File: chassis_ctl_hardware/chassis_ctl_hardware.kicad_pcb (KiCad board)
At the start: 2 copper layers, 75 x 75 mm, 53 parts, among them IC1 TJA1441AT, J1 USB_C, J2 Conn_01x05_Socket, J3 encoder1, J4 encoder2, J5 Conn_01x04_Socket, J6 RJ45, J7 STLink-v3mini, SW1 SW_Push, U1 BU33SD5WG-TR, U2 ICM-40609-D, U3 STM32U545CET6, Y1 16M

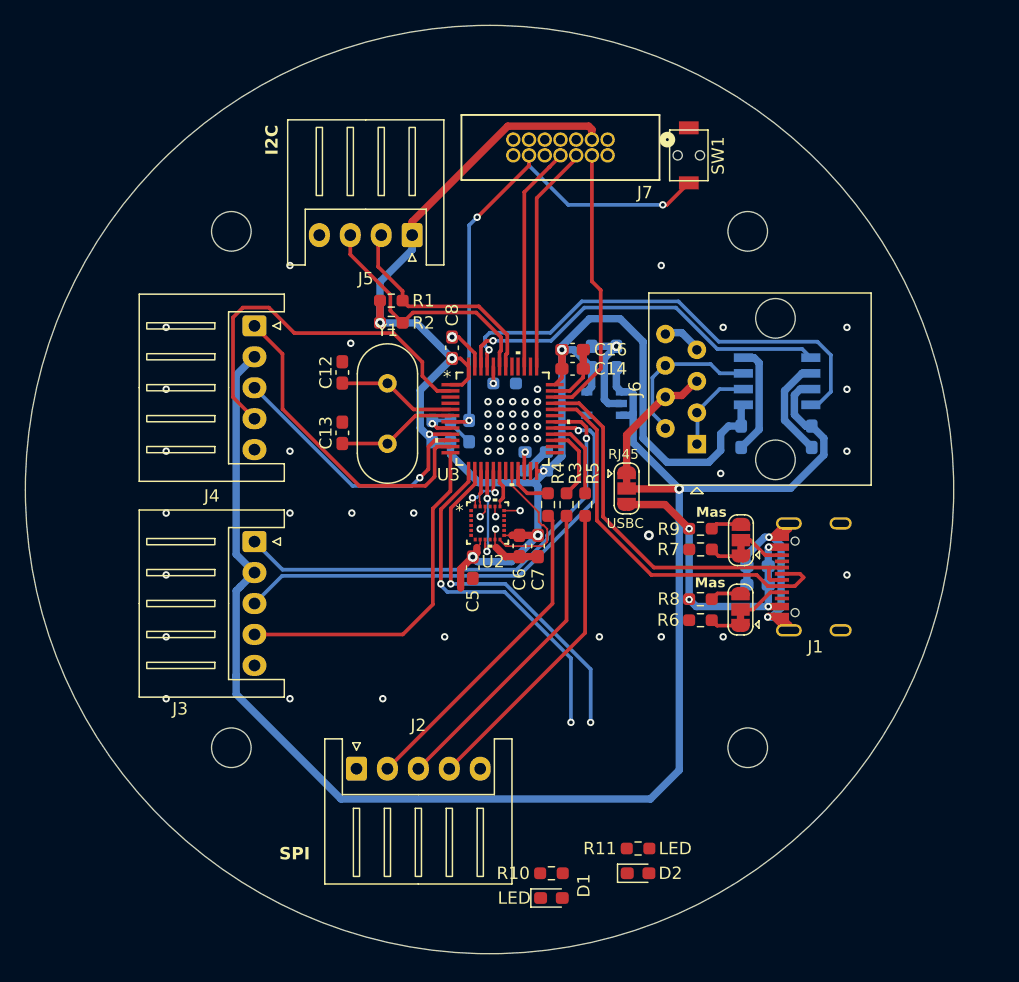
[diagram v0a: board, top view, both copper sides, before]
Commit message: Second_Commit
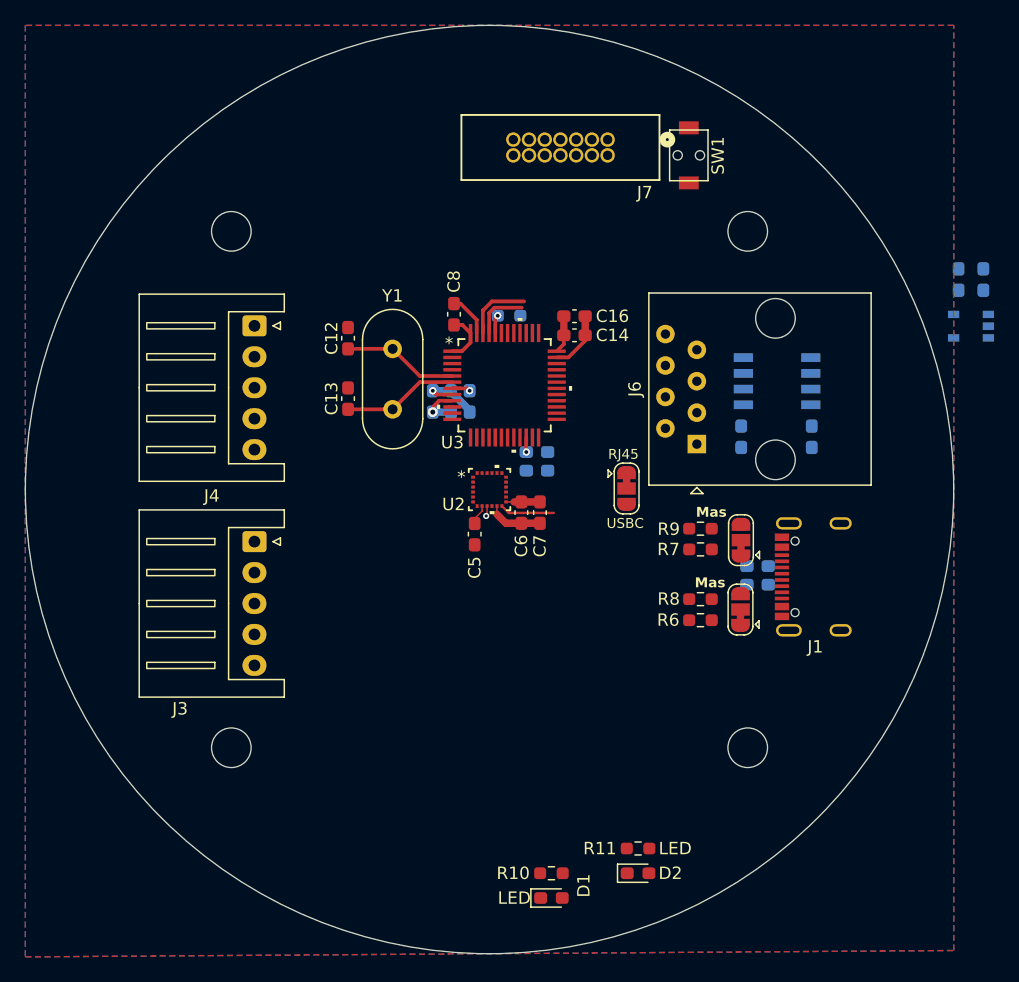
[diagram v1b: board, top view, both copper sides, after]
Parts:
- removed J2: Conn_01x05_Socket, Connector_JST:JST_XH_S5B-XH-A_1x05_P2.50mm_Horizontal
- removed J5: Conn_01x04_Socket, Connector_JST:JST_XH_S4B-XH-A_1x04_P2.50mm_Horizontal
- removed R1, R2: 4.7k, Resistor_SMD:R_0603_1608Metric_Pad0.98x0.95mm_HandSolder
- removed R3, R4, R5: 0, Resistor_SMD:R_0603_1608Metric_Pad0.98x0.95mm_HandSolder
- moved U1 30.3 mm to (199.4, 57.3)
- moved C3 30.3 mm to (198.4, 53.5)
- moved C4 30.3 mm to (200.4, 53.5)
- moved R12 5.48 mm to (162.1, 56.4)
- moved Y1 2.81 mm to (152.7, 64.0)
- moved C13 2.80 mm to (149.1, 63.1)
- moved C12 2.80 mm to (149.1, 58.3)
- moved C14 2.71 mm to (167.4, 58.0)
- moved C5 2.71 mm to (159.3, 74.1)
- moved U2 2.71 mm to (160.5, 70.5)
- moved C16 2.71 mm to (167.4, 56.5)
- moved C8 2.71 mm to (157.6, 56.3)
- moved U3 2.71 mm to (161.7, 62.1)
- moved C6 2.70 mm to (163.1, 72.3)
- moved C7 2.70 mm to (164.6, 72.3)
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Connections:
- net /TIM1_ETR renamed /TIM2_CH3
- J3 pad 1: /TIM1_CH2 -> /TIM2_CH2
- J3 pad 3: /TIM1_CH1 -> /TIM2_CH1
- J4 pad 1: /TIM2_CH2 -> /TIM3_CH2
- J4 pad 3: /TIM2_CH1 -> /TIM3_CH1
- J4 pad 4: /TIM2_ETR -> /TIM3_CH3
- U3 pad 13: /MCU/MCU_State_LED -> unconnected-(U3-PA3-Pad13)
- U3 pad 14: /MCU/FDCAN_State -> unconnected-(U3-PA4-Pad14)
- U3 pad 15: /IMU/SPI_CLK -> unconnected-(U3-PA5-Pad15)
- U3 pad 16: /IMU/SPI_MISO -> /TIM3_CH1
- U3 pad 17: /IMU/SPI_MOSI -> /TIM3_CH2
- U3 pad 18: /IMU/INT2/FSYNC -> /TIM3_CH3
- U3 pad 19: unconnected-(U3-PB1-Pad19) -> /MCU/MCU_State_LED
- U3 pad 2: /TIM2_ETR -> unconnected-(U3-PC13-Pad2)
- U3 pad 20: /IMU/INT1 -> /MCU/FDCAN_State
- U3 pad 21: /SPI2_SCK -> /IMU/SPI_CLK
- U3 pad 25: unconnected-(U3-PB12-Pad25) -> GND
- U3 pad 27: /SPI2_MISO -> /IMU/SPI_MISO
- U3 pad 28: /SPI2_MOSI -> /IMU/SPI_MOSI
- U3 pad 29: /TIM1_CH1 -> /IMU/INT2/FSYNC
- U3 pad 30: /TIM1_CH2 -> /IMU/INT1
- U3 pad 42: /I2C1_SCL -> unconnected-(U3-PB6-Pad42)
- U3 pad 43: /I2C1_SDA -> unconnected-(U3-PB7-Pad43)
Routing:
- net +5V: track 130.5 -> 0.00 mm, vias 1 -> 0
- net +3.3V: track 128.7 -> 15.1 mm, vias 7 -> 1
- net GND: track 73.4 -> 18.2 mm, vias 60 -> 1
- net /TIM1_CH1: track 39.7 -> 0.00 mm, vias 1 -> 0
- net /MCU/NRST: track 40.8 -> 1.47 mm, vias 3 -> 1
- net /TIM1_CH2: track 38.7 -> 0.00 mm, vias 1 -> 0
- net /FDCAN_Transceiver/CAN_RX: track 38.5 -> 4.44 mm, vias 1 -> 0
- net /D-: track 32.5 -> 0.00 mm
- net /TIM2_ETR: track 30.2 -> 0.00 mm
- net /D+: track 30.1 -> 0.00 mm
- net /MCU/MCU_State_LED: track 28.4 -> 0.00 mm, vias 2 -> 0
- net /MCU/FDCAN_State: track 28.4 -> 0.00 mm, vias 2 -> 0
- net /TIM2_CH3: track 28.3 -> 0.00 mm
- net /TIM2_CH2: track 26.4 -> 0.00 mm
- net Net-(J2-Pin_2): track 26.1 -> 0.00 mm
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- added copper zone on B.Cu, net GND
- added copper zone on F.Cu, net GND
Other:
- board text removed: "I2C"
- board text removed: "SPI"
